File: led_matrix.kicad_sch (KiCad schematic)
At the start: 119 parts, among them J1 I2C, J2 Extra, J3 Address, J4 +5V, J5 GND, J6 Power Input, J7 Columns, J8 Row Addr., J9 VCC, Q1 2N3904, Q2 2N3904, Q3 2N3904, Q4 2N3904, Q5 2N3904, Q6 2N3904, Q7 2N3904, Q8 2N3904, U1 MCP23017, U2 74AC245, U3 74HC238, U4 UA78M33CKCS

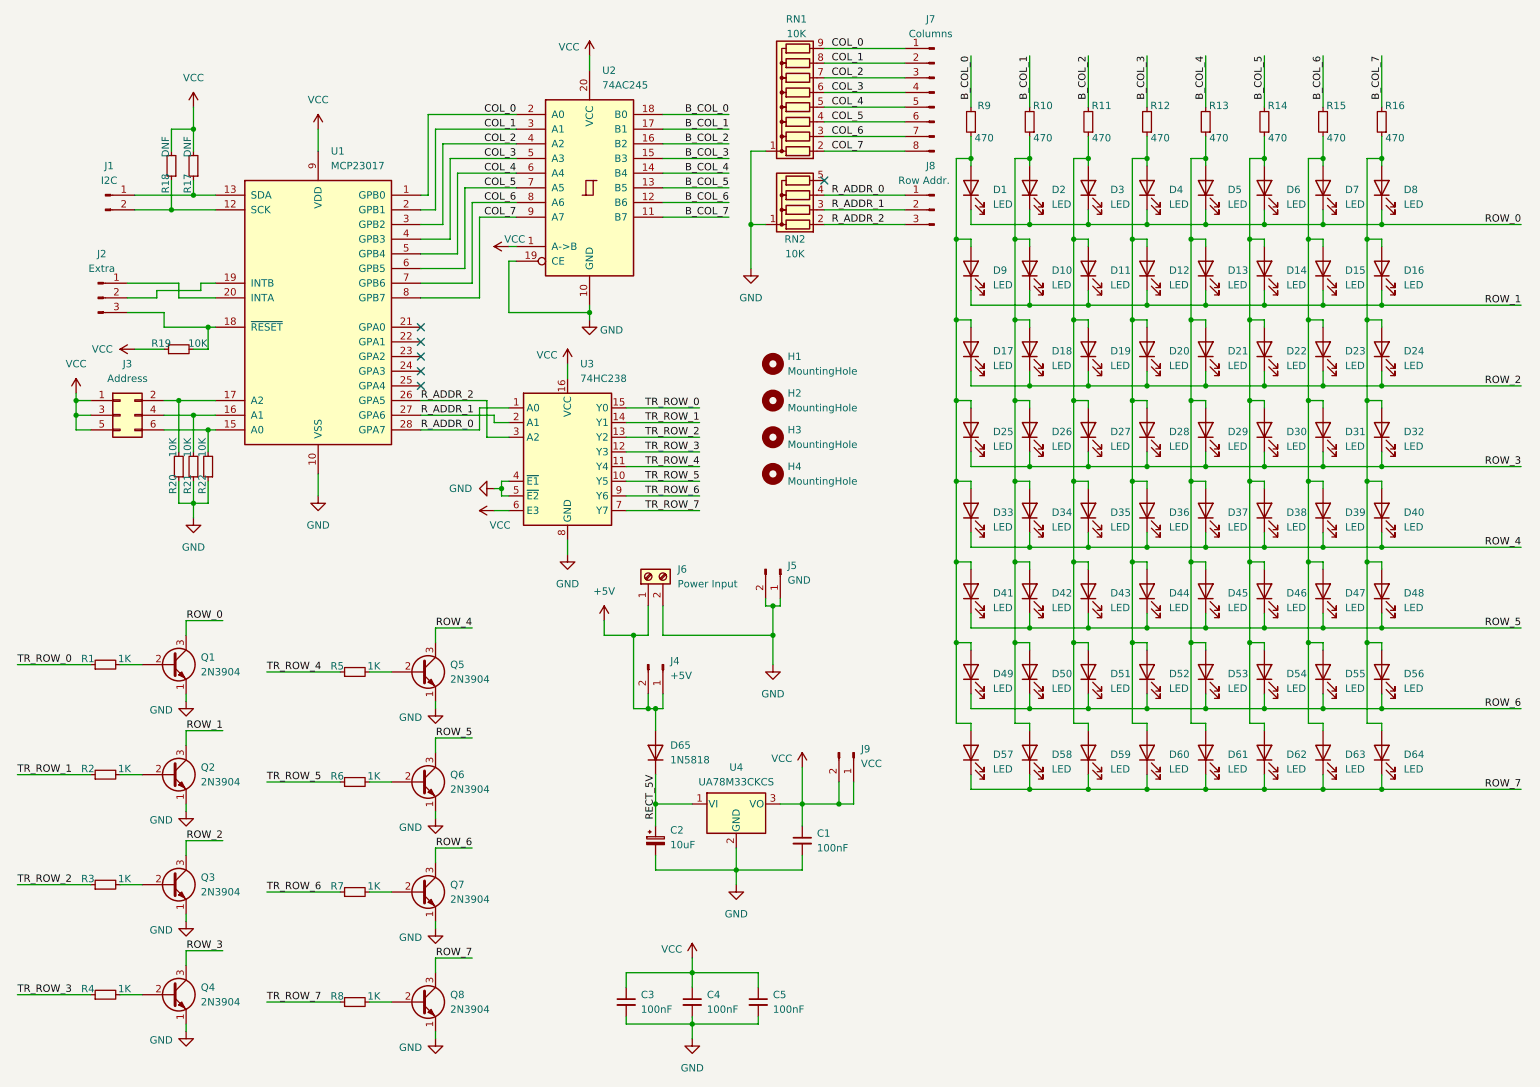
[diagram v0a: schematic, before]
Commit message: Updated readme
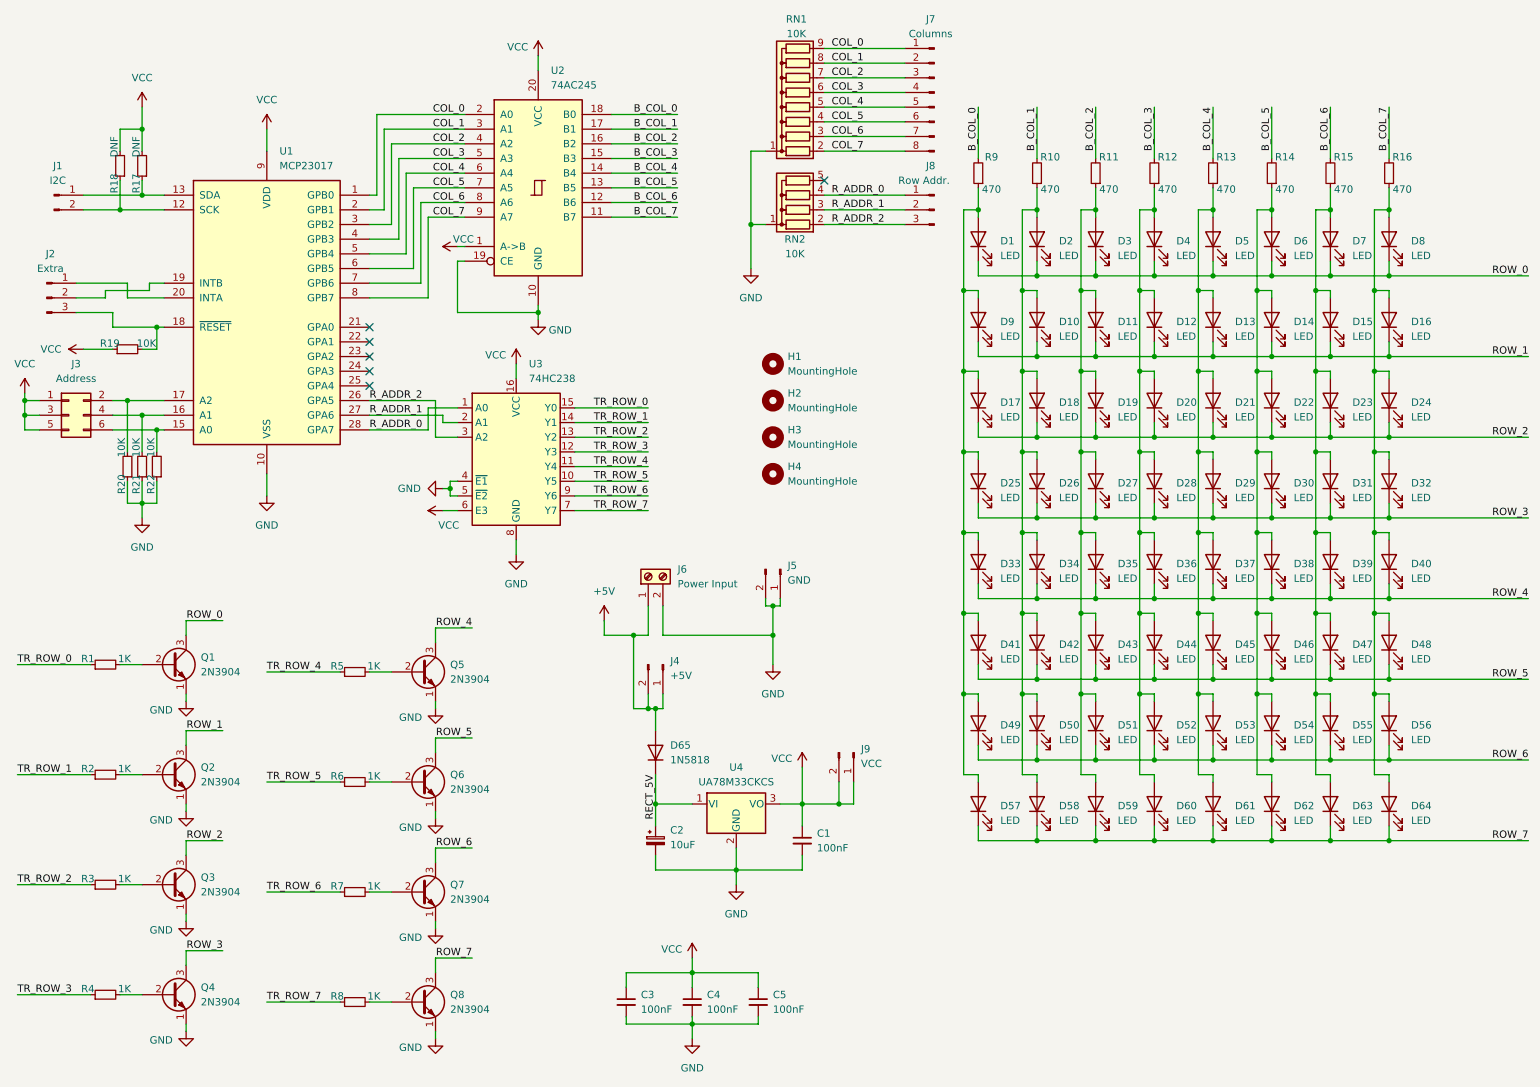
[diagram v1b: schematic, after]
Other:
- title: (none) -> 8x8 LED MATRIX EDUBOARD
- moved on the sheet: D1, D10, D11, D12, D13, D14, D15, D16, D17, D18, D19, D2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
